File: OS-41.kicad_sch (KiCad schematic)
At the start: 66 parts, among them J1 Conn_02x03_Counter_Clockwise, J2 Conn_01x02_Pin, J3 Conn_01x02_Pin, J4 Conn_Coaxial, J5 Conn_01x03, SW4 SW_Push, U1 BME280, U2 SI4432-B1-FMR, U3 MCP1640x-xCHY, U4 ATGM336H-5N31, U7 STM32F103C8Tx, Y1 32.768KHz 12.5pF, Y2 8MHz 12pF, Y3 30MHz 10pF

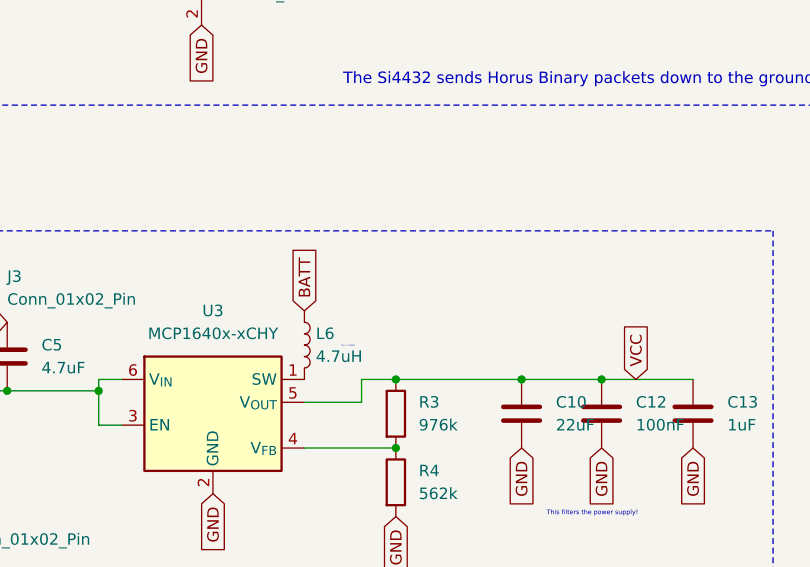
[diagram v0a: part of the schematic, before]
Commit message: add notice
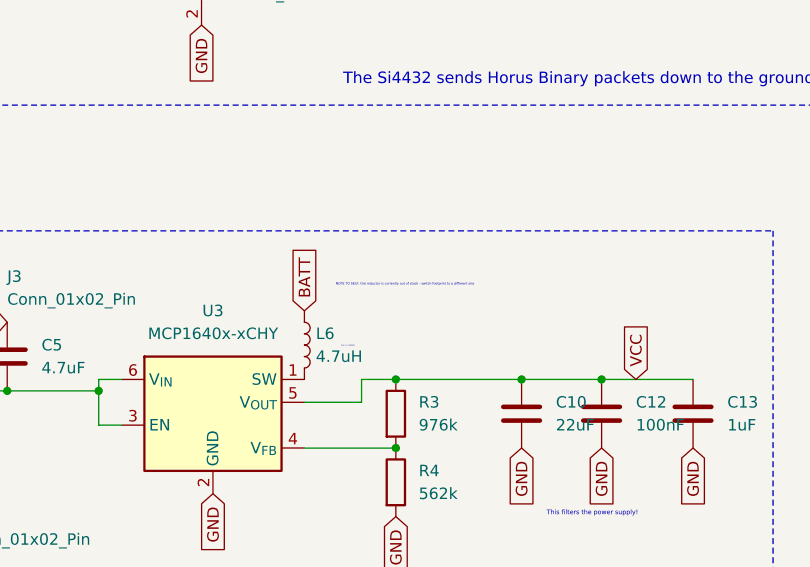
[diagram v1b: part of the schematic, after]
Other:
- note added: "NOTE TO SELF: this inductor is currently out of stock - switch footprint to a different one"
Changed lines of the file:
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@@
+		)
+	)
+	(text "NOTE TO SELF: this inductor is currently out of stock - switch footprint to a different one"
+		(exclude_from_sim no)
+		(at 96.266 221.996 0)
+		(effects
+			(font
+				(size 0.254 0.254)
+			)
 		)
 	)
